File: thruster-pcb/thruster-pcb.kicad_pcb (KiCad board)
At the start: 4 copper layers, 60 x 160 mm, 163 parts, among them J1001 Connector_USB_C_Receptacle_US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, J1101 Connector_USB_C_Receptacle_US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, J501 Connector_USB_C_Receptacle_US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, J601 Connector_USB_C_Receptacle_US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, J701 Connector_USB_C_Receptacle_US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, J801 Connector_USB_C_Receptacle_US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, J901 Connector_USB_C_Receptacle_US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, SW1201 SW_DIP_x08_SDA08H1SBDR, T301 TERM_BLK_HDR_2POS_90DEG_0.2IN, U1001 LTC6820HMS-TRPBF, U1002 TPS1H200AQDGNRQ1, U1003 Buffer_74LVC1G125DRYR, U1101 LTC6820HMS-TRPBF, U1102 TPS1H200AQDGNRQ1, U1103 Buffer_74LVC1G125DRYR, U1201 TCA6408ARGTR, U1401 TPA6204A1DRBR, U301 TPSM365R6V5RDNR, U501 LTC6820HMS-TRPBF, U502 TPS1H200AQDGNRQ1, U503 Buffer_74LVC1G125DRYR, U601 LTC6820HMS-TRPBF, U602 TPS1H200AQDGNRQ1, U603 Buffer_74LVC1G125DRYR, U701 LTC6820HMS-TRPBF, U702 TPS1H200AQDGNRQ1, U703 Buffer_74LVC1G125DRYR, U801 LTC6820HMS-TRPBF, U802 TPS1H200AQDGNRQ1, U803 Buffer_74LVC1G125DRYR, U901 LTC6820HMS-TRPBF, U902 TPS1H200AQDGNRQ1, U903 Buffer_74LVC1G125DRYR

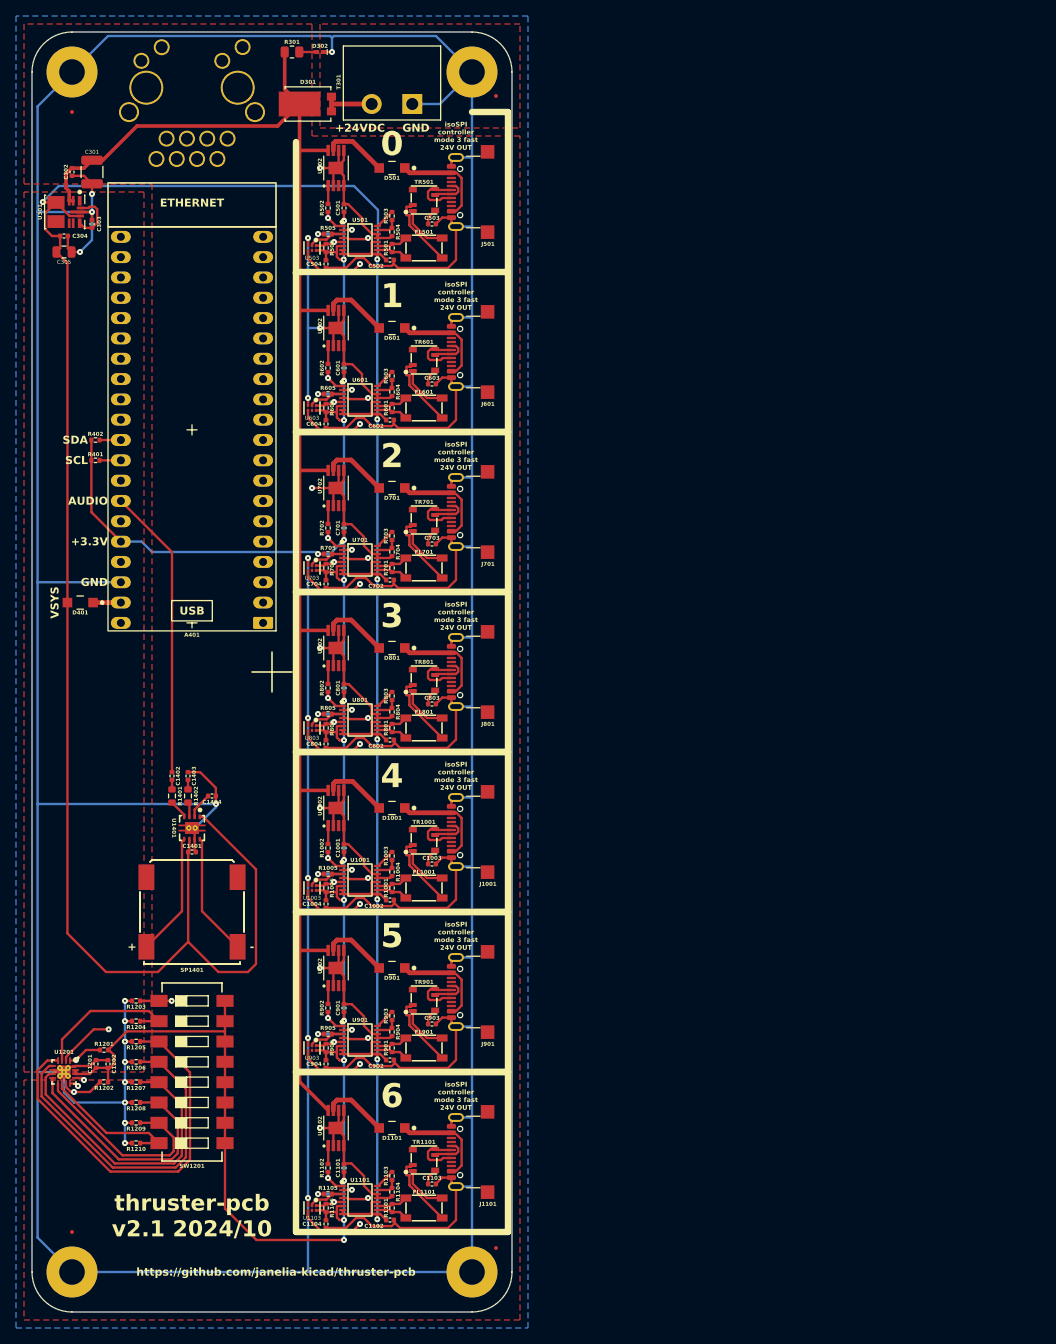
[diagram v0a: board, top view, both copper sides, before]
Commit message: Initial schematic and layout
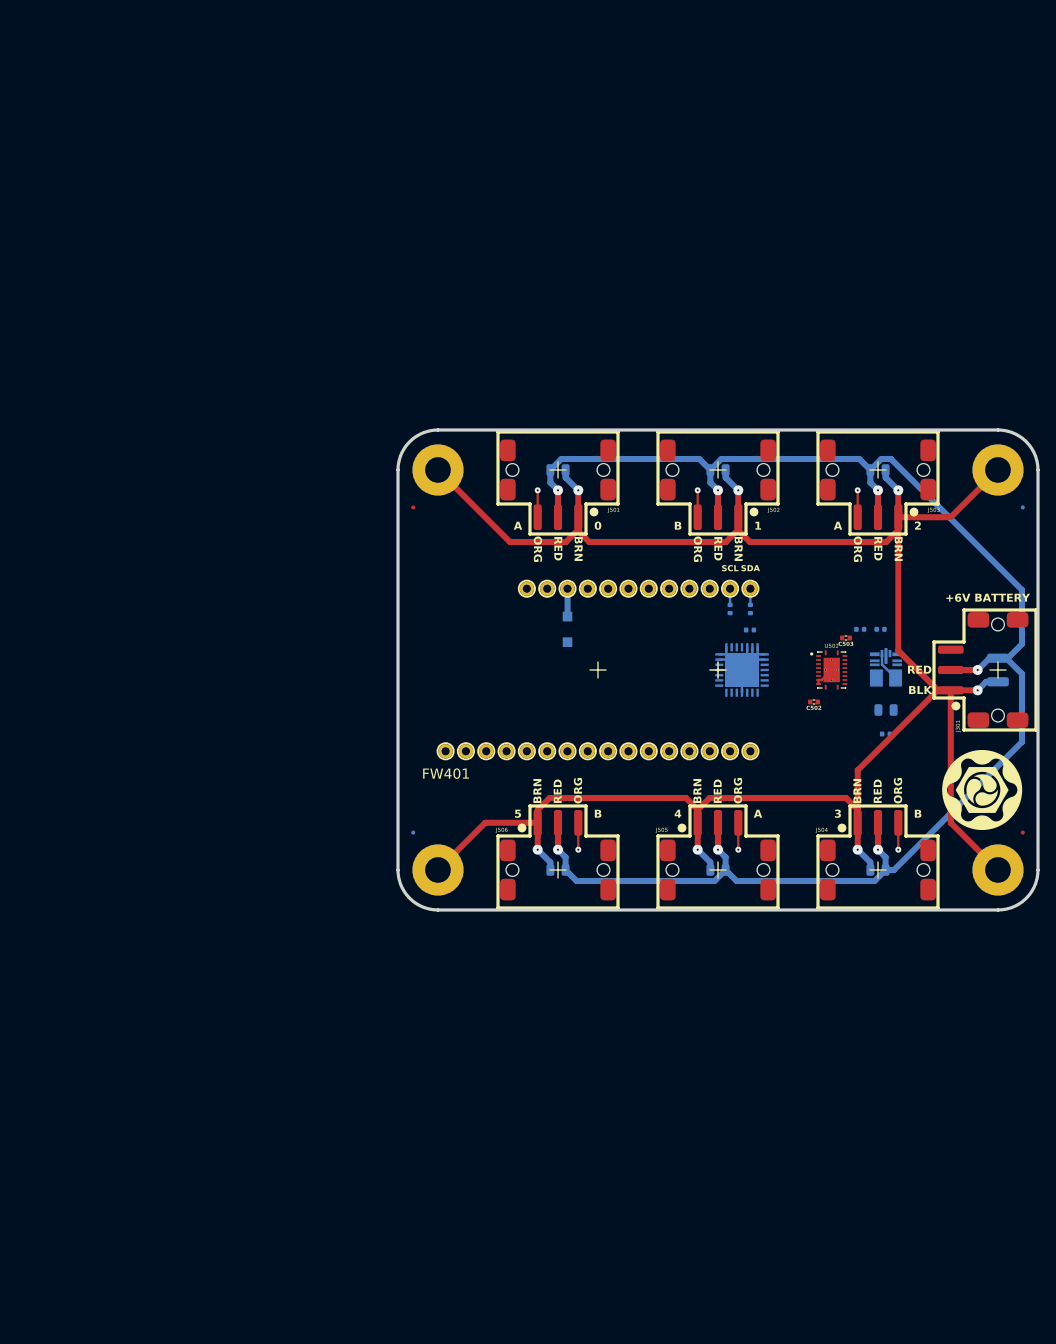
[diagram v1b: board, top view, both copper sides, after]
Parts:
- removed A401: PICO_W5500_EVB, Janelia:Pico-W5500-EVB_Header_Holes
- removed C1001, C1002, C1004, C1101, C1102, C1104, C1201, C1202, C601, C602, C604, C701, C702, C704, C801, C802, C804, C901, C902, C904: 0.1uF_100V, Janelia:C_0402_1005Metric
- removed C1003, C1103, C603, C703, C803, C903: 27pF_50V, Janelia:C_0402_1005Metric
- removed C1401: 1uF_35V, Janelia:C_0402_1005Metric
- removed C1402, C1403, C1404: 0.22uF_25V, Janelia:C_0402_1005Metric
- removed D1001, D1101, D501, D601, D701, D801, D901: D_SCHOTTKY_20V_1A, Janelia:SOD-123FL
- removed D301: D_50V_15A, Janelia:POWERDI5_DIO
- removed D302: LED_RED, Janelia:LED_0402-1005_KNB
- removed FL1001, FL1101, FL501, FL601, FL701, FL801, FL901: Choke_CMF_ACT45B-220-2P, Janelia:SMD_0-2P-TL003_TDK-L
- removed J1001, J1101, J601, J701, J801, J901: Connector_USB_C_Receptacle_USB2.0_16P_GT-USB-7047C, Janelia:USB_C_Receptacle_GT-USB-7047C_16P_TopMnt_Horizontal
- removed R1001, R1101, R501, R601, R701, R801, R901: 100, Janelia:R_0402_1005Metric
- removed R1002, R1102, R502, R602, R702, R802, R902: 4.7k, Janelia:R_0402_1005Metric
- removed R1003, R1103, R503, R603, R703, R803, R903: 1.4k, Janelia:R_0402_1005Metric
- removed R1004, R1104, R504, R604, R704, R804, R904: 604, Janelia:R_0402_1005Metric
- removed R1005, R1006, R1105, R1106, R505, R506, R605, R606, R705, R706, R805, R806, R905, R906: 1.8k, Janelia:R_0402_1005Metric
- removed R1201, R1202, R1203, R1204, R1205, R1206, R1207, R1208, R1209, R1210: 10.0k, Janelia:R_0402_1005Metric
- removed R1401, R1402: 40k, Janelia:R_0603_1608Metric
- removed R301: 2.32k, Janelia:R_0805_2012Metric
- removed SP1401: Speaker_13x13mm_8Ohm_700mW, Janelia:Speaker_13x13mm_KLJ-01304T-08R07W
- removed SW1201: SW_DIP_x08_SDA08H1SBDR, Janelia:SW_DIP_SPSTx08_Slide_SDA08H1SBDR
- removed T301: TERM_BLK_HDR_2POS_90DEG_0.2IN, Janelia:PHOENIX_1757242
- removed TR1001, TR1101, TR501, TR601, TR701, TR801, TR901: 1:1, Janelia:FB020G00
- removed U1001, U1101, U601, U701, U801, U901: LTC6820HMS-TRPBF, Janelia:MS_05-08-1669_ADI
- removed U1002, U1102, U602, U702, U802, U902: TPS1H200AQDGNRQ1, Janelia:SOP65P490X110-9N
- removed U1003, U1103, U503, U603, U703, U803, U903: Buffer_74LVC1G125DRYR, Janelia:DRY6
- removed U1201: TCA6408ARGTR, Janelia:QFN50P300X300X100-17N
- removed U1401: TPA6204A1DRBR, Janelia:DRB8_1P75X1P5
- added C505: 47uF_10V, Janelia:C_0805_2012Metric, B.Cu at (158.2, 76.3)
- added C506: 47uF_10V, Janelia:C_0805_2012Metric, B.Cu at (178.2, 76.3)
- added C507: 47uF_10V, Janelia:C_0805_2012Metric, B.Cu at (178.2, 126.3)
- added C508: 47uF_10V, Janelia:C_0805_2012Metric, B.Cu at (158.2, 126.3)
- added C509: 47uF_10V, Janelia:C_0805_2012Metric, B.Cu at (138.2, 126.3)
- added FW401: FEATHERWING_nRF52_HEADERS, Janelia:FEATHERWING_HEADERS, F.Cu at (143.2, 101.3)
- added G101: LOGO-10mm, MechatronicMagicLogo:logo-white-fg-black-bg-10mm, F.Cu at (191.2, 116.3)
- added J301: Conn_TERM_HDR_01x03_Pin_3.5mm_Horizontal, Janelia:Connector_Header_1x03_P2.54mm_Horizontal_SMD_284052-E, F.Cu at (193.2, 101.3)
- added J502: Conn_TERM_HDR_01x03_Pin_3.5mm_Horizontal, Janelia:Connector_Header_1x03_P2.54mm_Horizontal_SMD_284052-E, F.Cu at (158.2, 76.3)
- added J503: Conn_TERM_HDR_01x03_Pin_3.5mm_Horizontal, Janelia:Connector_Header_1x03_P2.54mm_Horizontal_SMD_284052-E, F.Cu at (178.2, 76.3)
- added J504: Conn_TERM_HDR_01x03_Pin_3.5mm_Horizontal, Janelia:Connector_Header_1x03_P2.54mm_Horizontal_SMD_284052-E, F.Cu at (178.2, 126.3)
- added J505: Conn_TERM_HDR_01x03_Pin_3.5mm_Horizontal, Janelia:Connector_Header_1x03_P2.54mm_Horizontal_SMD_284052-E, F.Cu at (158.2, 126.3)
- added J506: Conn_TERM_HDR_01x03_Pin_3.5mm_Horizontal, Janelia:Connector_Header_1x03_P2.54mm_Horizontal_SMD_284052-E, F.Cu at (138.2, 126.3)
- C301, C302, C303, C304, C305, C501, D401, FID202, FID204, R401, R402, U301: moved to B.Cu
- C503: value 27pF_50V -> 0.1uF_100V
- C504: value 0.1uF_100V -> 47uF_10V; footprint Janelia:C_0402_1005Metric -> Janelia:C_0805_2012Metric; moved to B.Cu
- J501: value Connector_USB_C_Receptacle_USB2.0_16P_GT-USB-7047C -> Conn_TERM_HDR_01x03_Pin_3.5mm_Horizontal; footprint Janelia:USB_C_Receptacle_GT-USB-7047C_16P_TopMnt_Horizontal -> Janelia:Connector_Header_1x03_P2.54mm_Horizontal_SMD_284052-E
- U501: value LTC6820HMS-TRPBF -> PCA9685BS; footprint Janelia:MS_05-08-1669_ADI -> Janelia:QFN-28-1EP_6x6mm_P0.65mm_EP4.25x4.25mm; moved to B.Cu
- U502: value TPS1H200AQDGNRQ1 -> LevelTranslator_TXS0108EPW; footprint Janelia:SOP65P490X110-9N -> Janelia:IC_TXS0108ERGYR
- moved C301 129.2 mm to (193.2, 101.3)
- moved C304 120.1 mm to (179.2, 109.3), turned to 180 degrees
- moved C305 117.6 mm to (179.2, 106.3), turned to 180 degrees
- moved U301 117.6 mm to (179.2, 101.3), turned to 180 degrees
- moved C302 116.1 mm to (178.5, 96.3), turned to 180 degrees
- moved C303 108.6 mm to (175.9, 96.3), turned to 0 degrees
- moved U502 88.2 mm to (172.4, 101.3), turned to 0 degrees
- moved R402 84.5 mm to (162.2, 93.7), turned to 90 degrees
- moved FID203 83.9 mm to (196.2, 121.7)
- moved FID202 83.6 mm to (196.2, 81.0), turned to 180 degrees
- moved H203 82.8 mm to (193.2, 126.3)
- moved H202 82.5 mm to (193.2, 76.3)
- moved R401 81.5 mm to (159.7, 93.7), turned to 90 degrees
- moved C502 76.6 mm to (170.2, 105.3), turned to 180 degrees
- moved C501 73.2 mm to (162.2, 96.3), turned to 0 degrees
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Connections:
- C301 pad 1: /VAA -> /+6V
- C302 pad 1: /VAA -> /+6V
- C502 pad 1: /+5V -> /+3.3V
- C503 pad 1: /prism-0/CT -> /+5V
- C504 pad 1: /+3.3V -> /+6V
- D401 pad 1: /microcontroller/VSYS -> /microcontroller/VBUS
- U301 pad 2: /VAA -> /+6V
- U301 pad 3: /VAA -> /+6V
- U501 pad 1: /~{PRISMS_RESET} -> /GND
- U501 pad 10: /prism-0/I2- -> unconnected-(U501-LED7-Pad10)
- U501 pad 11: /prism-0/I2+ -> /GND
- U501 pad 12: /+5V -> unconnected-(U501-LED8-Pad12)
- U501 pad 13: /GND -> unconnected-(U501-LED9-Pad13)
- U501 pad 14: /GND -> unconnected-(U501-LED10-Pad14)
- U501 pad 15: /prism-0/ICMP -> unconnected-(U501-LED11-Pad15)
- U501 pad 16: /prism-0/IBIAS -> unconnected-(U501-LED12-Pad16)
- U501 pad 2: /PRISM_COPI -> /GND
- U501 pad 3: /prism-0/CIPO_UNBUFFERED -> /thrusters/PWM_0
- U501 pad 4: /PRISM_SCK -> /thrusters/PWM_1
- U501 pad 5: /~{PRISM_CS_0} -> /thrusters/PWM_2
- U501 pad 6: /+3.3V -> /thrusters/PWM_3
- U501 pad 7: /+5V -> /thrusters/PWM_4
- U501 pad 8: /+5V -> /thrusters/PWM_5
- U501 pad 9: /+5V -> unconnected-(U501-LED6-Pad9)
- U502 pad 1: Net-(U502-IN) -> /thrusters/PWM_0
- U502 pad 2: /GND -> /+3.3V
- U502 pad 3: unconnected-(U502-~{FAULT}-Pad3) -> /thrusters/PWM_1
- U502 pad 4: /GND -> /thrusters/PWM_2
- U502 pad 5: /GND -> /thrusters/PWM_3
- U502 pad 6: /GND -> /thrusters/PWM_4
- U502 pad 7: /prism-0/VBB -> /thrusters/PWM_5
- U502 pad 8: /VAA -> /GND
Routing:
- net /GND: track 1037.9 -> 295.4 mm, vias 27 -> 7
- net /+5V: track 401.7 -> 3.75 mm, vias 8 -> 0
- net /+3.3V: track 319.9 -> 0.00 mm, vias 22 -> 0
- net /+6V: track 0.00 -> 201.6 mm, vias 0 -> 7
- net /PRISM_CIPO: track 195.6 -> 0.00 mm, vias 7 -> 0
- net /VAA: track 193.0 -> 0.00 mm
- net /PRISM_SCK: track 157.1 -> 0.00 mm, vias 7 -> 0
- net /~{PRISMS_RESET}: track 150.0 -> 0.00 mm, vias 7 -> 0
- net /PRISM_COPI: track 143.6 -> 0.00 mm, vias 7 -> 0
- net /~{PRISM_CS_6}: track 89.7 -> 0.00 mm, vias 1 -> 0
- net /SDA: track 86.4 -> 2.03 mm, vias 1 -> 0
- net /SCL: track 84.9 -> 2.03 mm, vias 1 -> 0
- net /~{ADDRESS_INT}: track 78.9 -> 0.00 mm, vias 1 -> 0
- net /~{PRISM_CS_5}: track 72.3 -> 0.00 mm, vias 1 -> 0
- net /~{ADDRESS_RESET}: track 68.6 -> 0.00 mm, vias 1 -> 0
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- removed copper zone on F.Cu, net /+5V
- removed copper zone on B.Cu, net /GND
- removed copper zone on In1.Cu, net /GND
- removed copper zone on In2.Cu, net /GND
- removed copper zone on F.Cu, net /VAA
- removed copper zone on F.Cu, net /power/VAA
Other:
- board size 60 x 160 mm -> 80 x 60 mm
- board text removed: "+24VDC"
- board text removed: "+3.3V"
- board text removed: "0"
- board text removed: "1"
- board text removed: "2"
- board text removed: "3"
- board text removed: "4"
- board text removed: "5"
- board text removed: "6"
- board text removed: "AUDIO"
- board text removed: "GND"
- board text removed: "VSYS"
- board text removed: "https://github.com/janelia-kicad/thruster-pcb"
- board text removed: "isoSPI controller mode 3 fast 24V OUT"
- board text removed: "thruster-pcb v2.1 2024/10"
